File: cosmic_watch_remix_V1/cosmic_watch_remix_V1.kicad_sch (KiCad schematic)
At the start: 21 parts, among them IC1 MICROFJ-60035-TSV-TR1, J1 Conn_01x05_Female, U1 ADS1115IDGS

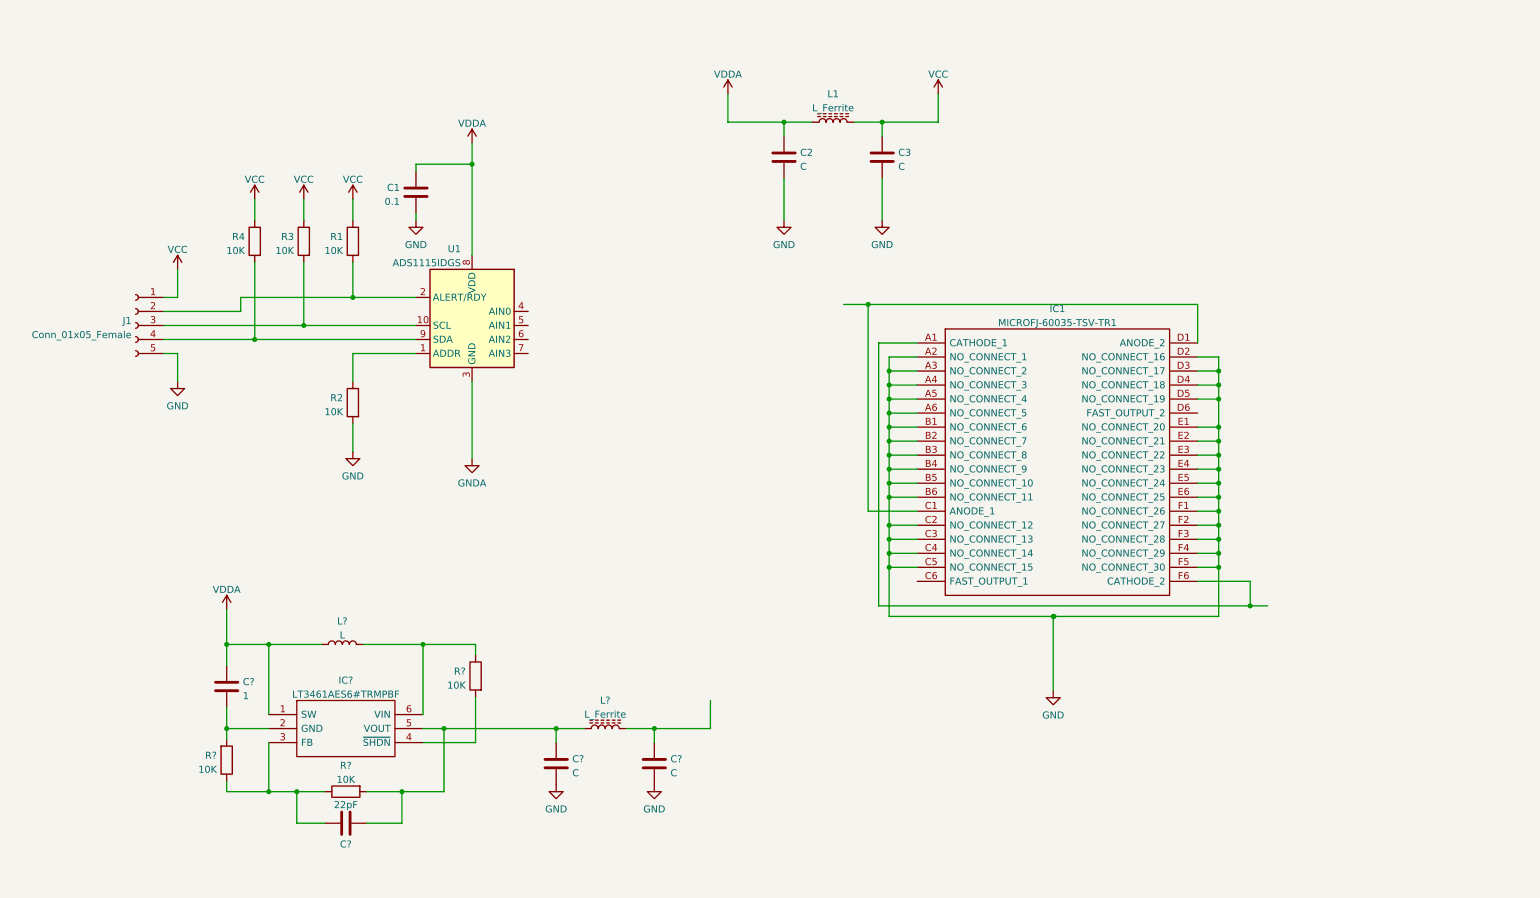
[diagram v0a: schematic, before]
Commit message: Component Initial Layout Complete
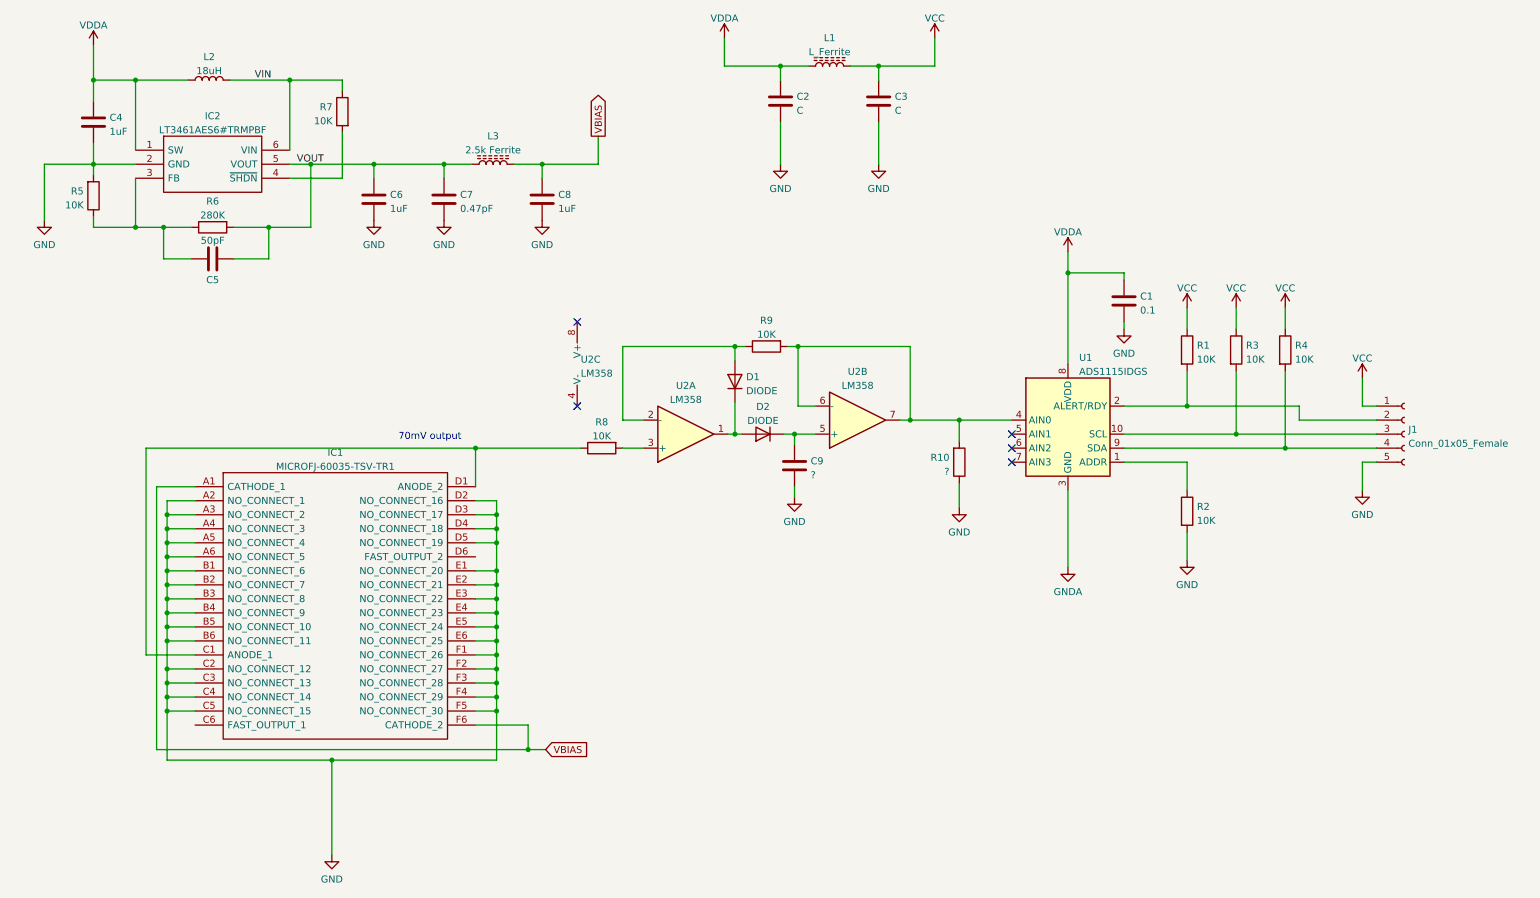
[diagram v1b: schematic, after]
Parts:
- added C6: 1uF, Capacitor_SMD:C_0603_1608Metric, symbol Device:C
- added C9: ?, Capacitor_SMD:C_0603_1608Metric, symbol Device:C
- added D1, D2: DIODE, Diode_SMD:D_SOD-323, symbol Simulation_SPICE:DIODE
- added R10: ?, Resistor_SMD:R_0603_1608Metric, symbol Device:R
- added R8, R9: 10K, Resistor_SMD:R_0603_1608Metric, symbol Device:R
- added U2: LM358, Package_SO:SOIC-8_7.5x5.85mm_P1.27mm, symbol Amplifier_Operational:LM358
- C2, C3: footprint (none) -> Capacitor_SMD:C_0603_1608Metric
- C4: renamed from C?; value 1 -> 1uF
- C5: renamed from C?; value 22pF -> 50pF; footprint (none) -> Capacitor_SMD:C_0603_1608Metric
- C7: renamed from C?; value C -> 0.47pF; footprint (none) -> Capacitor_SMD:C_0603_1608Metric
- C8: renamed from C?; value C -> 1uF; footprint (none) -> Capacitor_SMD:C_0603_1608Metric
- IC1: footprint MICROFJ60035TSVTR1 -> SiPM:MICROFJ60035TSVTR1
- IC2: renamed from IC?; footprint SOT95P280X100-6N -> Package_TO_SOT_SMD:TSOT-23-6
- L1: footprint (none) -> Resistor_SMD:R_0603_1608Metric
- L2: renamed from L?; value L -> 18uH; footprint (none) -> Inductor_SMD:L_1210_3225Metric
- L3: renamed from L?; value L_Ferrite -> 2.5k Ferrite; footprint (none) -> Resistor_SMD:R_0603_1608Metric
- R6: renamed from R?; value 10K -> 280K
- gave numbers to parts that had none: 2
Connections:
- net GND: now also C4.2, IC1.D2 (NO_CONNECT_16), IC1.D3 (NO_CONNECT_17), IC1.D4 (NO_CONNECT_18), IC1.D5 (NO_CONNECT_19), IC1.E1 (NO_CONNECT_20), IC1.E2 (NO_CONNECT_21), IC1.E3 (NO_CONNECT_22), IC1.E4 (NO_CONNECT_23), IC1.E5 (NO_CONNECT_24), IC1.E6 (NO_CONNECT_25), IC1.F1 (NO_CONNECT_26), IC1.F2 (NO_CONNECT_27), IC1.F3 (NO_CONNECT_28), IC1.F4 (NO_CONNECT_29), IC1.F5 (NO_CONNECT_30), IC2.2 (GND), R5.2, C6.2, C9.2, R10.1
- net VOUT: now reaches C5.1, C7.1, IC2.5 (VOUT), L3.1, R6.2
- net VOUT: now also C6.1
- net VIN: now reaches IC2.6 (VIN), L2.2, R7.1
- net VBIAS: now reaches C8.1, L3.2
- net VBIAS: now also IC1.A1 (CATHODE_1), IC1.F6 (CATHODE_2)
- net at U1.4 (AIN0): now also R10.2, R9.2, U2.6 (-), U2.7
- net at IC1.C1 (ANODE_1), IC1.D1 (ANODE_2): now also R8.1
- new net: D1.1 (A), R9.1, U2.2 (-)
- new net: D1.2 (K), D2.1 (A), U2.1
- new net: R8.2, U2.3 (+)
- new net: C9.1, D2.2 (K), U2.5 (+)
- no-connect marks 0 -> 5
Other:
- note added: "70mV output"
- moved on the sheet: C1, C2, C3, C4, C5, C7, C8, IC1, IC2, J1, L1, L2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
